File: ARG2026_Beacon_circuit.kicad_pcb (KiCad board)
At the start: 2 copper layers, 100 x 86.6 mm, 30 parts, among them J1 Conn_01x02_Pin, J2 Conn_01x02_Pin, Q1 IRLML0030, SW1 SW_SPDT, U1 CH32V002A4M6

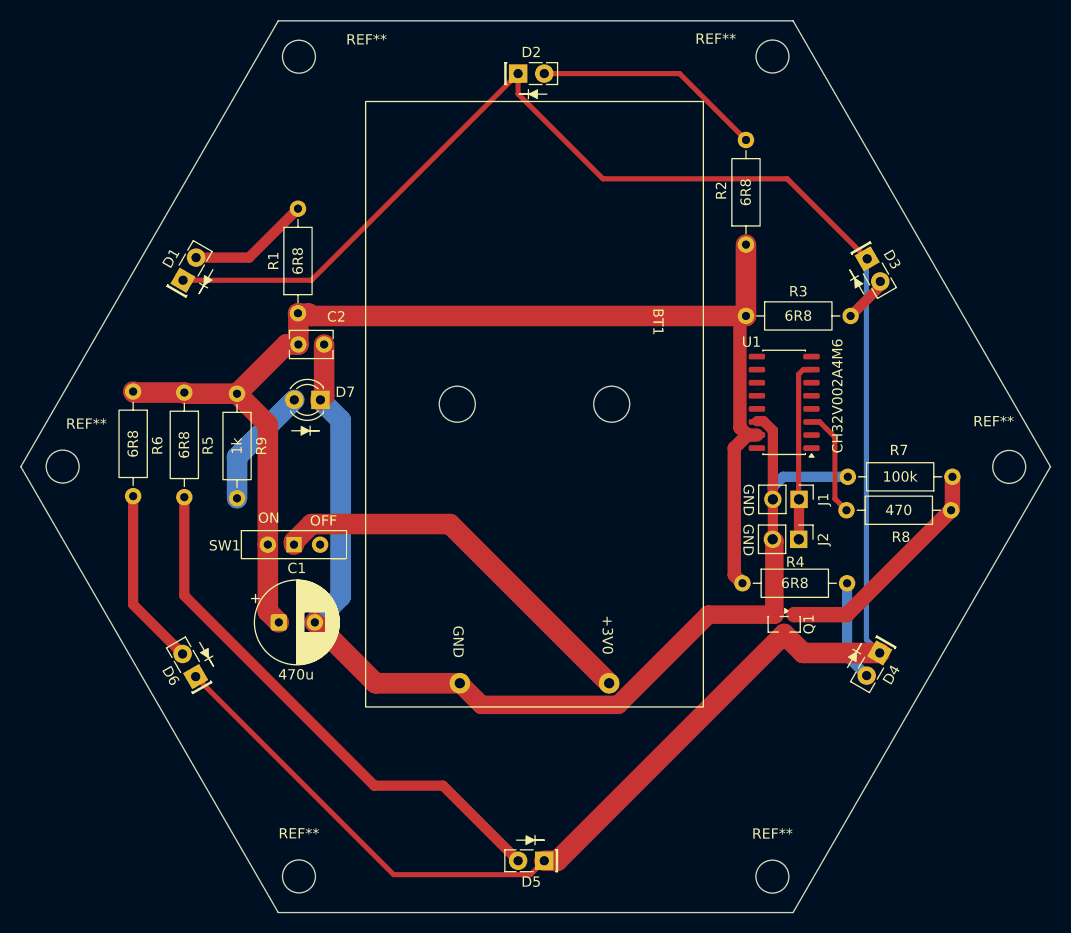
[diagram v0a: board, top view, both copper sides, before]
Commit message: GND塗りつぶしを忘れてました
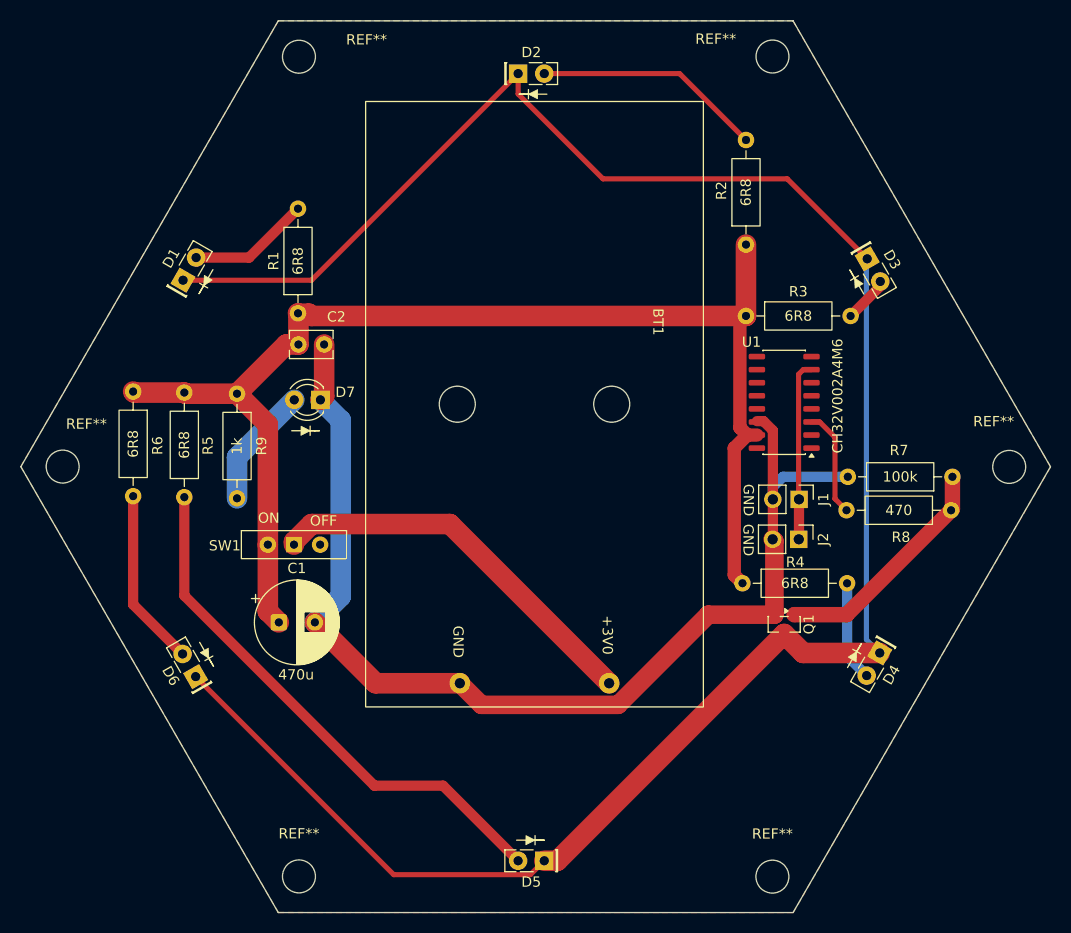
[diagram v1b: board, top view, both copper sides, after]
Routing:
- added copper zone on F.Cu, net GND
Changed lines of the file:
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@@
+	)
+	(zone
+		(net "GND")
+		(layer "F.Cu")
+		(hatch edge 0.5)
+		(connect_pads
+			(clearance 0.5)
+		)
+		(min_thickness 0.25)
+		(fill yes
+			(thermal_gap 0.5)
+			(thermal_bridge_width 0.5)
+			(island_removal_mode 0)
+		)
+		(polygon
+			(pts
+				(xy 196.07 57.81) (xy 246.05 57.81) (xy 271.07 101.13) (xy 246.07 144.42) (xy 196.07 144.41) (xy 171.06 101.098086)
+			)
+		)
 	)
 	(zone
